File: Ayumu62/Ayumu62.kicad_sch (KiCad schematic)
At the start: 11 parts, among them U1 YAAJ_BluePill

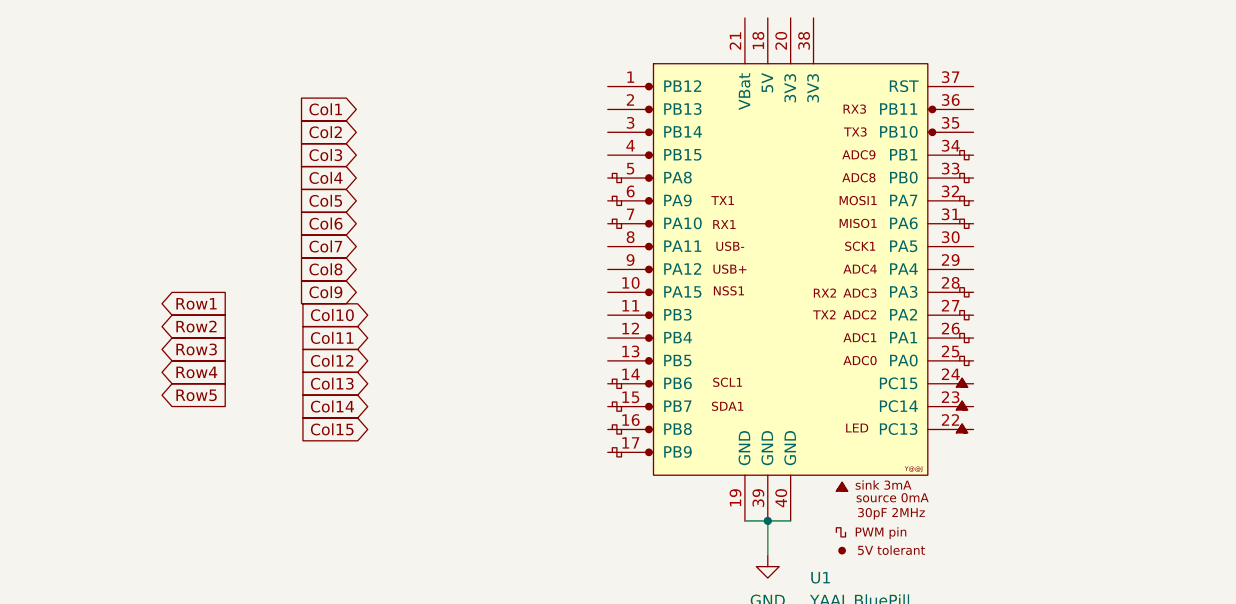
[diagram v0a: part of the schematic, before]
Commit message: upd
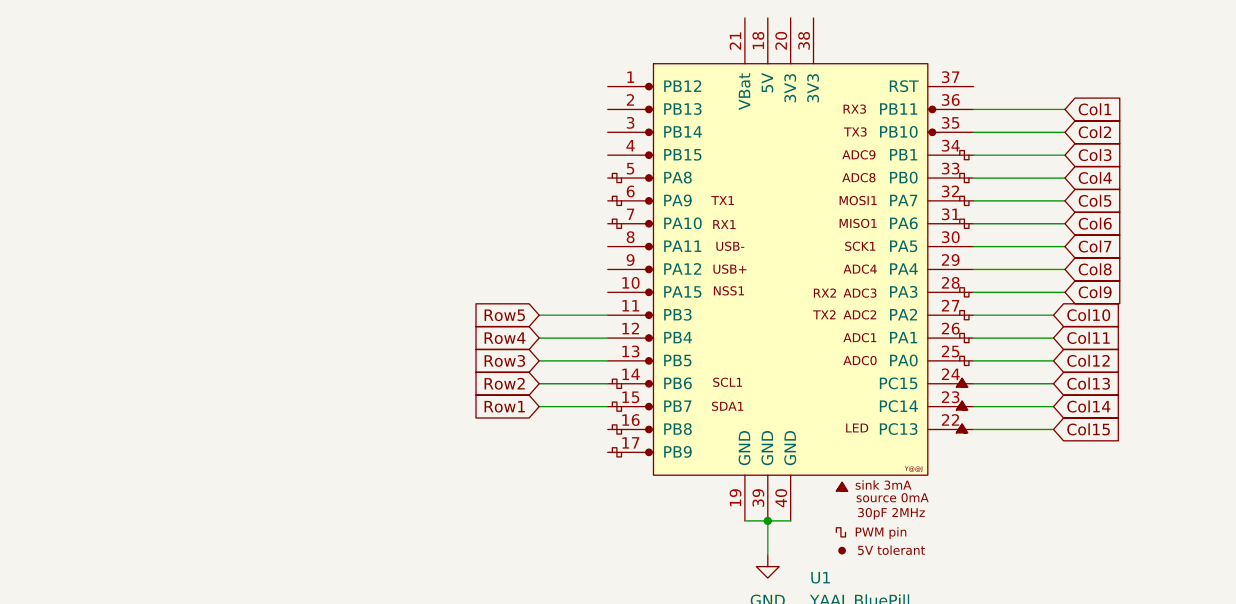
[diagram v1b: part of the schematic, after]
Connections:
- net Col1: now also U1.36 (PB11)
- net Col10: now also U1.27 (PA2)
- net Col11: now also U1.26 (PA1)
- net Col12: now also U1.25 (PA0)
- net Col13: now also U1.24 (PC15)
- net Col14: now also U1.23 (PC14)
- net Col15: now also U1.22 (PC13)
- net Col2: now also U1.35 (PB10)
- net Col3: now also U1.34 (PB1)
- net Col4: now also U1.33 (PB0)
- net Col5: now also U1.32 (PA7)
- net Col6: now also U1.31 (PA6)
- net Col7: now also U1.30 (PA5)
- net Col8: now also U1.29 (PA4)
- net Col9: now also U1.28 (PA3)
- net Row1: now also U1.15 (PB7)
- net Row2: now also U1.14 (PB6)
- net Row3: now also U1.13 (PB5)
- net Row4: now also U1.12 (PB4)
- net Row5: now also U1.11 (PB3)

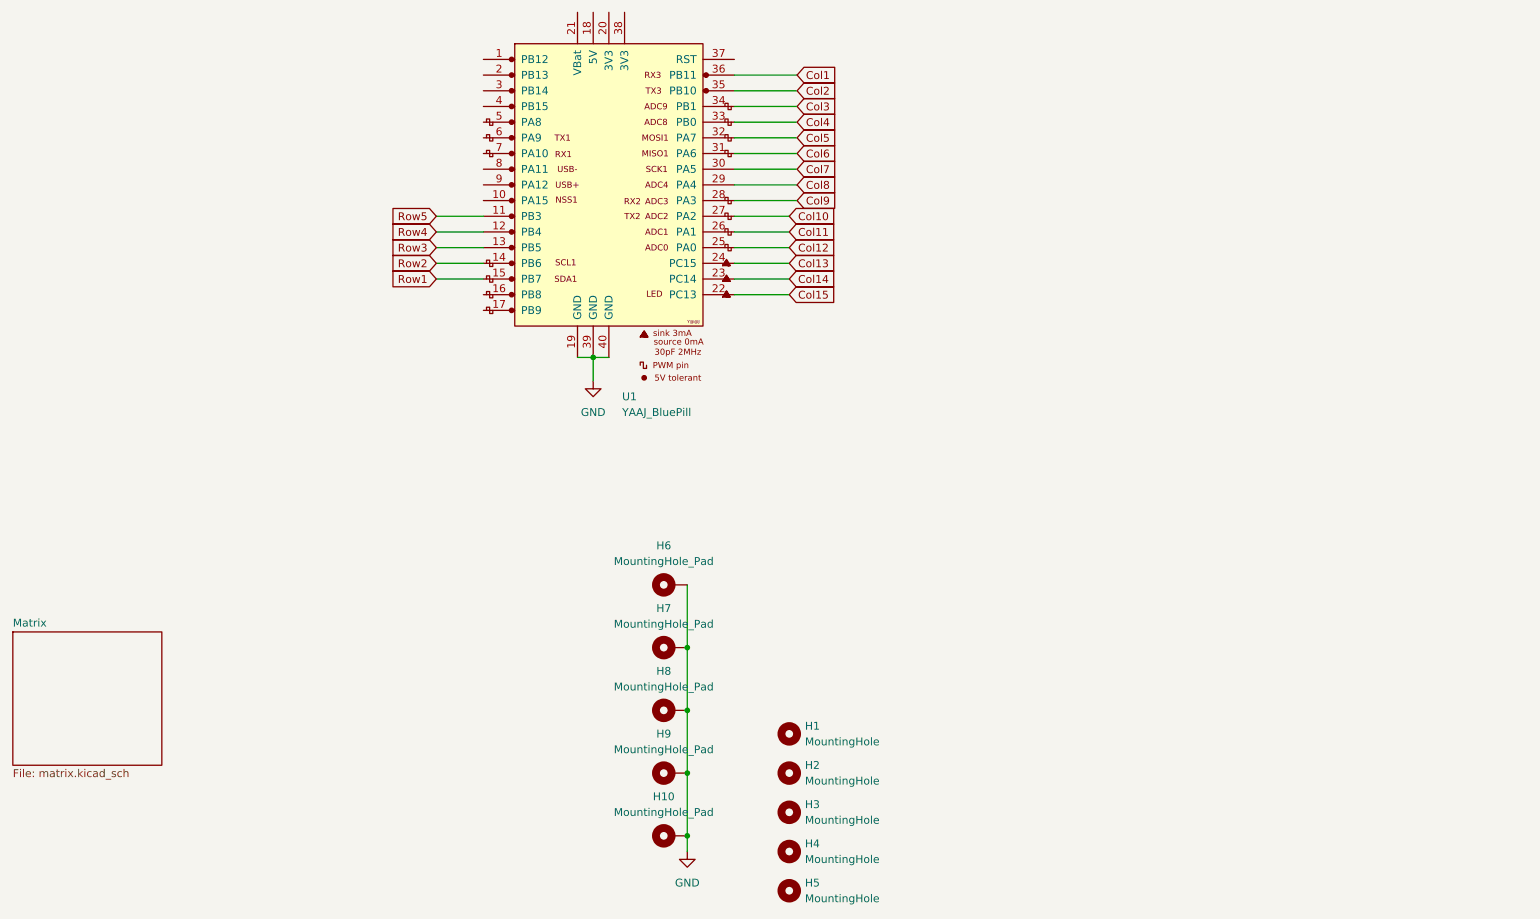
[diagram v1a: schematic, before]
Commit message: upd
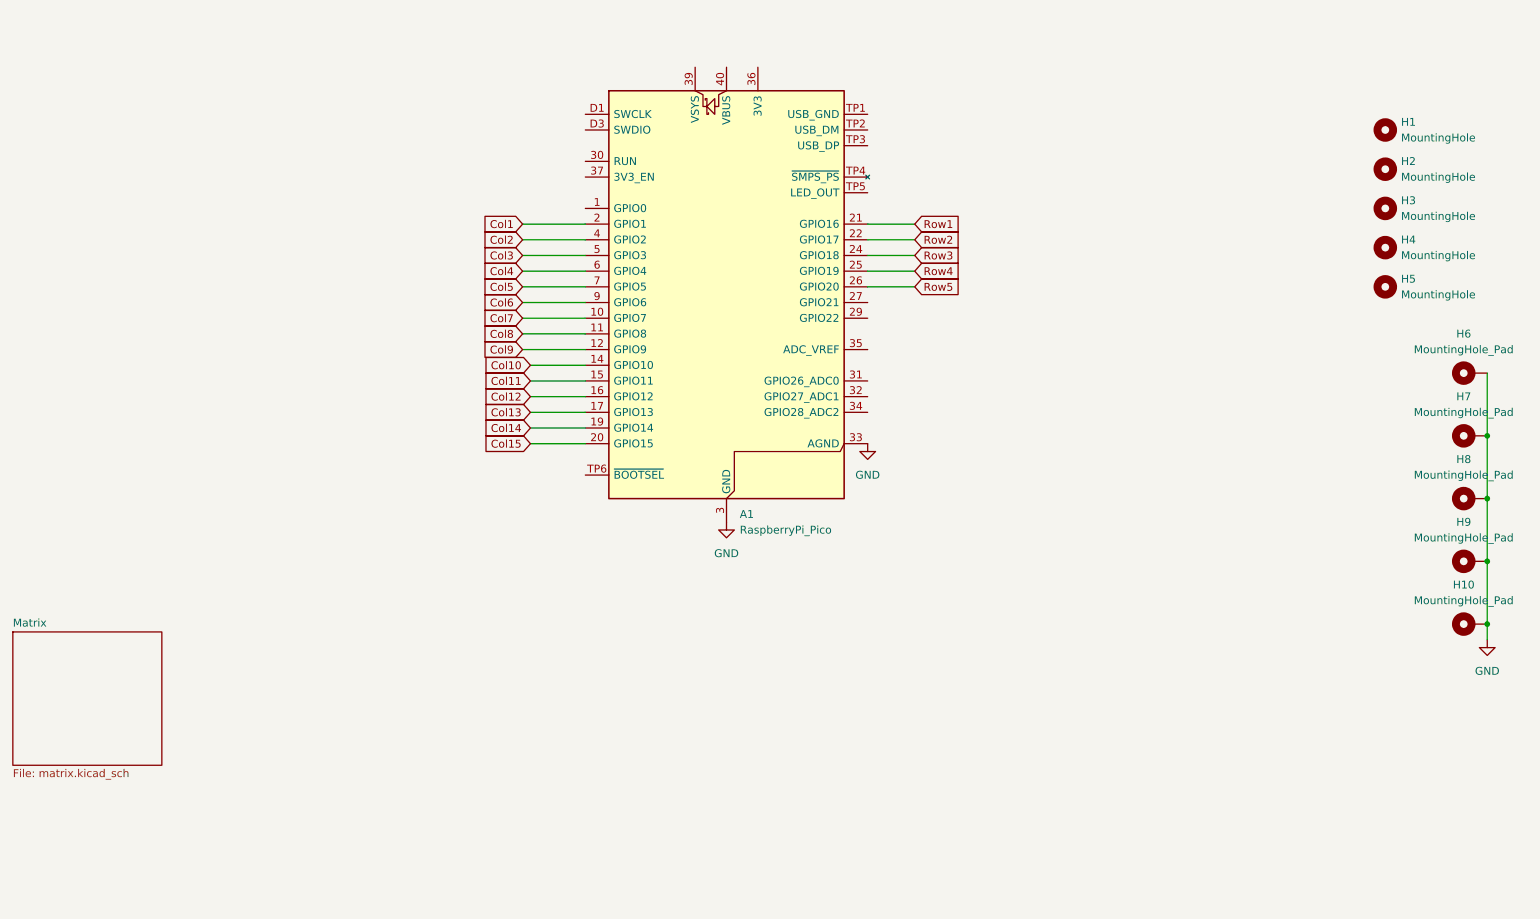
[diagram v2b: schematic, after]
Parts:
- removed U1: YAAJ_BluePill, YAAJ:YAAJ_BluePill_2, symbol Zero.countersteer:YAAJ_BluePill
- added A1: RaspberryPi_Pico, Module:RaspberryPi_Pico_Common_Unspecified, symbol MCU_Module:RaspberryPi_Pico_Extensive
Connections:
- net Col1: now also A1.2 (GPIO1)
- net Col10: now also A1.14 (GPIO10)
- net Col11: now also A1.15 (GPIO11)
- net Col12: now also A1.16 (GPIO12)
- net Col13: now also A1.17 (GPIO13)
- net Col14: now also A1.19 (GPIO14)
- net Col15: now also A1.20 (GPIO15)
- net Col2: now also A1.4 (GPIO2)
- net Col3: now also A1.5 (GPIO3)
- net Col4: now also A1.6 (GPIO4)
- net Col5: now also A1.7 (GPIO5)
- net Col6: now also A1.9 (GPIO6)
- net Col7: now also A1.10 (GPIO7)
- net Col8: now also A1.11 (GPIO8)
- net Col9: now also A1.12 (GPIO9)
- net GND: now also A1.13 (GND), A1.18 (GND), A1.23 (GND), A1.28 (GND), A1.3 (GND), A1.33 (AGND), A1.38 (GND), A1.8 (GND), A1.D2 (GND)
- net Row1: now also A1.21 (GPIO16)
- net Row2: now also A1.22 (GPIO17)
- net Row3: now also A1.24 (GPIO18)
- net Row4: now also A1.25 (GPIO19)
- net Row5: now also A1.26 (GPIO20)
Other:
- moved on the sheet: H1, H10, H2, H3, H4, H5, H6, H7, H8, H9
